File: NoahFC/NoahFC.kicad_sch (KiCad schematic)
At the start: 35 parts, among them J1 ALE, J10 GND, J11 SCK, J12 MISO, J13 VCC, J14 GND, J15 A1, J16 A3, J17 D6, J18 RESET, J2 ELE, J3 MPU6050, J4 FTDI, J5 VCC, J6 THR, J7 PPM, J8 GPS, J9 A0, U1 ATmega328, U3 AMS1117-5.0, Y1 16Mhz

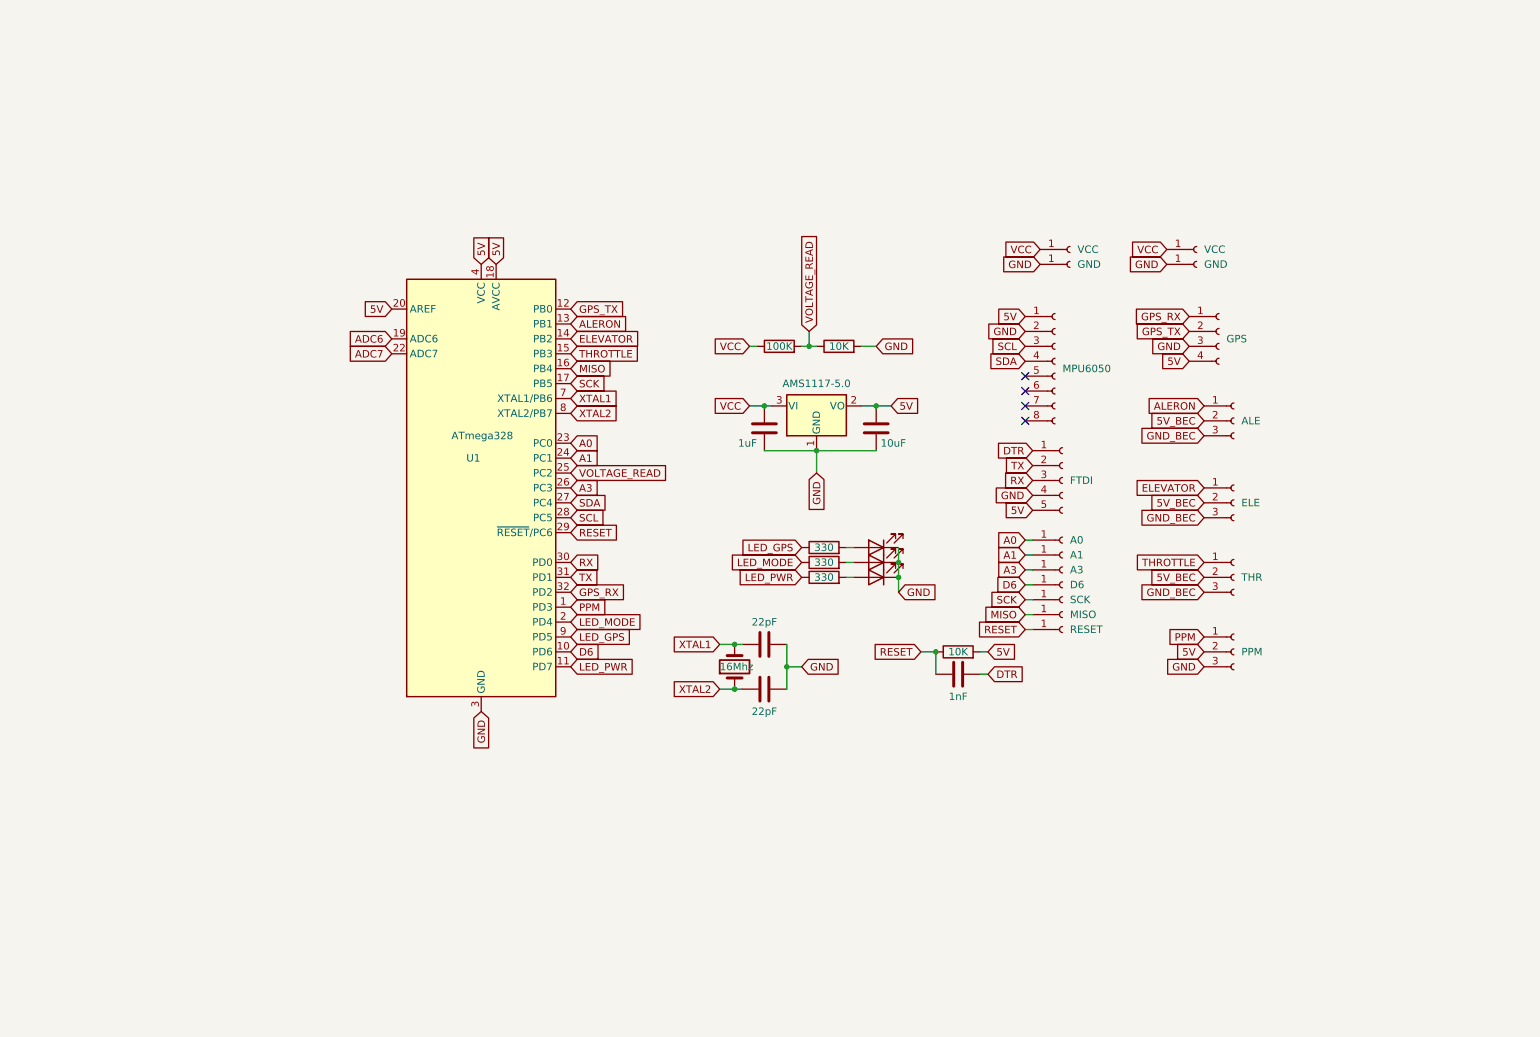
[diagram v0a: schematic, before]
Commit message: add rev2 version board
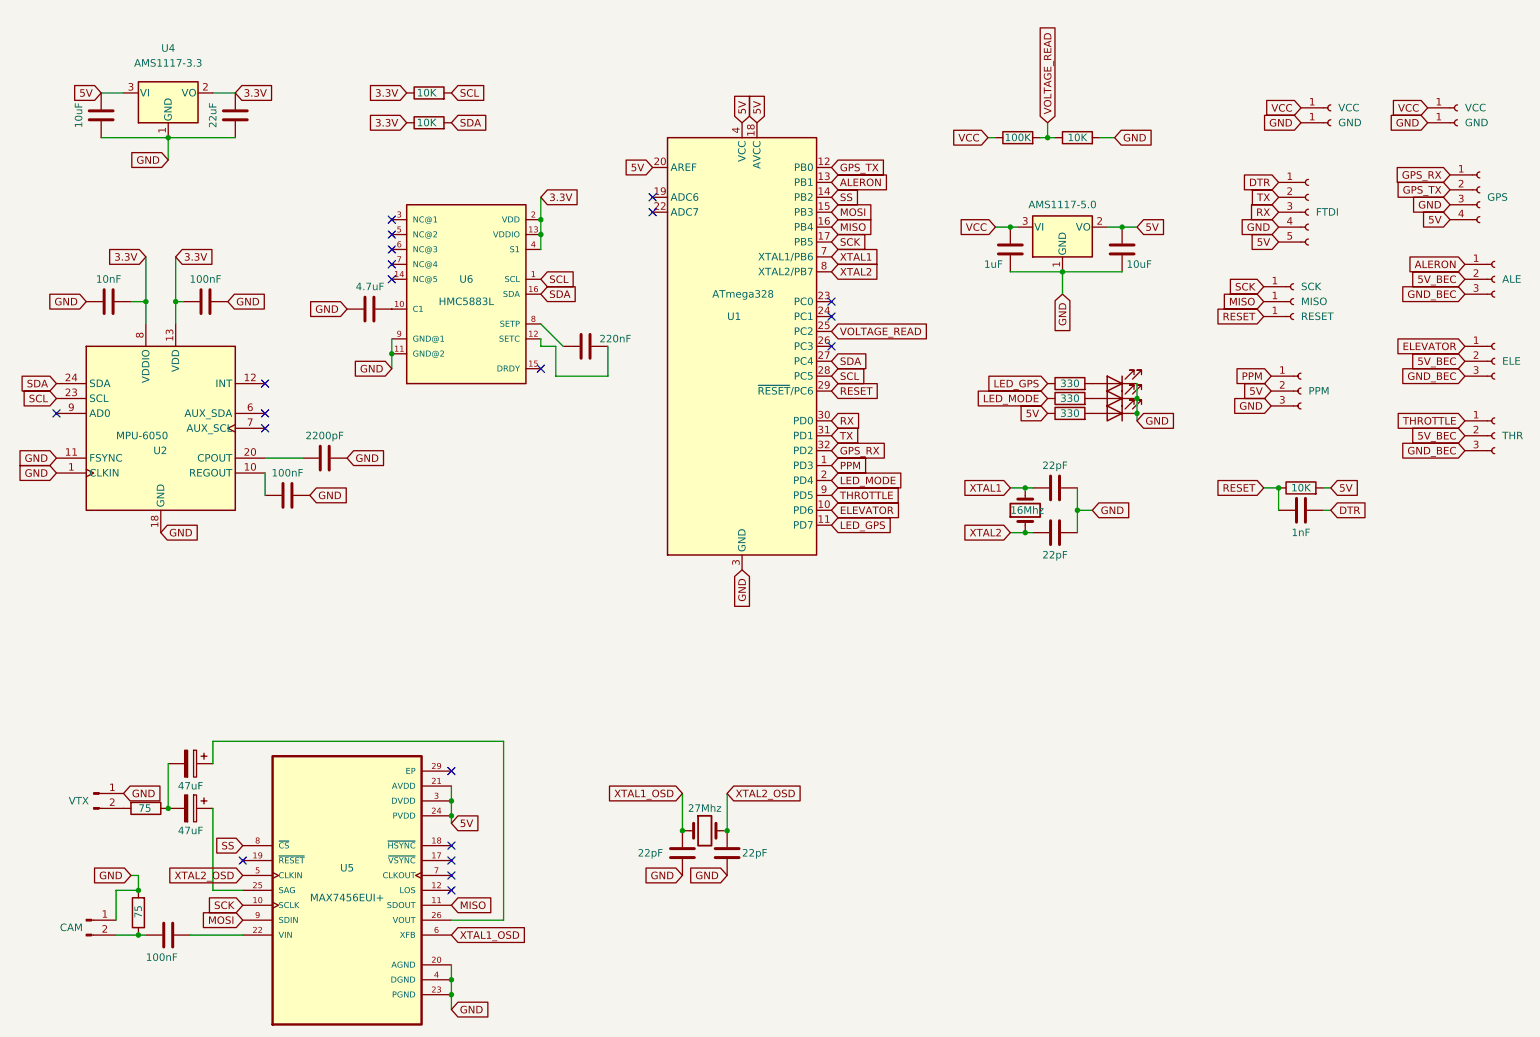
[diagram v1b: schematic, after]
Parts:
- removed J15: A1, TestPoint:TestPoint_Pad_1.0x1.0mm, symbol Connector:Conn_01x01_Female
- removed J16: A3, TestPoint:TestPoint_Pad_1.0x1.0mm, symbol Connector:Conn_01x01_Female
- removed J17: D6, TestPoint:TestPoint_Pad_1.0x1.0mm, symbol Connector:Conn_01x01_Female
- removed J3: MPU6050, Connector_PinHeader_2.54mm:PinHeader_1x08_P2.54mm_Vertical, symbol Connector:Conn_01x08_Female
- removed J9: A0, TestPoint:TestPoint_Pad_1.0x1.0mm, symbol Connector:Conn_01x01_Female
- added C10: 10uF, Capacitor_SMD:C_0805_2012Metric, symbol Device:C
- added C11: 22uF, Capacitor_SMD:C_0805_2012Metric, symbol Device:C
- added C12, C13: 22pF, Capacitor_SMD:C_0805_2012Metric, symbol Device:C
- added C17, C7, C8: 100nF, Capacitor_SMD:C_0805_2012Metric, symbol Device:C
- added C18, C19: 47uF, Capacitor_Tantalum_SMD:CP_EIA-3216-18_Kemet-A, symbol Device:C_Polarized
- added C20: 4.7uF, Capacitor_SMD:C_0805_2012Metric, symbol Device:C
- added C21: 220nF, Capacitor_SMD:C_0805_2012Metric, symbol Device:C
- added C6: 10nF, Capacitor_SMD:C_0805_2012Metric, symbol Device:C
- added C9: 2200pF, Capacitor_SMD:C_0805_2012Metric, symbol Device:C
- added J16: CAM, Connector_PinHeader_2.54mm:PinHeader_1x02_P2.54mm_Vertical, symbol Connector:Conn_01x02_Male
- added J17: VTX, Connector_PinHeader_2.54mm:PinHeader_1x02_P2.54mm_Vertical, symbol Connector:Conn_01x02_Male
- added R10, R9: 75, Resistor_SMD:R_0805_2012Metric, symbol Device:R
- added R7, R8: 10K, Resistor_SMD:R_0805_2012Metric, symbol Device:R
- added U2: MPU-6050, Sensor_Motion:InvenSense_QFN-24_4x4mm_P0.5mm, symbol Sensor_Motion:MPU-6050
- added U4: AMS1117-3.3, Package_TO_SOT_SMD:SOT-223-3_TabPin2, symbol Regulator_Linear:AP1117-33
- added U5: MAX7456EUI+, SOP65P637X110-28N, symbol MAX7456EUI_:MAX7456EUI+
- added U6: HMC5883L, LPCC-16, symbol HMC5883L:HMC5883L
- added Y2: 27Mhz, Crystal:Crystal_SMD_3225-4Pin_3.2x2.5mm, symbol Device:Crystal
- Y1: footprint Crystal:Crystal_SMD_HC49-SD -> Crystal:Crystal_SMD_3225-4Pin_3.2x2.5mm
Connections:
- net D6 is gone; now on net ELEVATOR: U1.10 (PD6)
- net 5V: now also R4.1, C10.2, U4.3 (VI), U5.21 (AVDD), U5.24 (PVDD), U5.3 (DVDD)
- net ELEVATOR: no longer U1.14 (PB2)
- net GND: now also C10.1, C11.1, C12.2, C13.2, C20.1, C6.1, C7.2, C8.2, C9.2, J16.1 (Pin_1), J17.1 (Pin_1), R9.2, U2.1 (CLKIN), U2.11 (FSYNC), U2.18 (GND), U4.1 (GND), U5.20 (AGND), U5.23 (PGND), U5.4 (DGND), U6.11 (GND@2), U6.9 (GND@1)
- net LED_GPS: now also U1.11 (PD7); no longer U1.9 (PD5)
- net MISO: now also U5.11 (SDOUT)
- net SCK: now also U5.10 (SCLK)
- net SCL: now also R7.2, U2.23 (SCL), U6.1 (SCL)
- net SDA: now also R8.2, U2.24 (SDA), U6.16 (SDA)
- net THROTTLE: now also U1.9 (PD5); no longer U1.15 (PB3)
- net A0: no longer names the net of U1.23 (PC0)
- net A1: no longer names the net of U1.24 (PC1)
- net A3: no longer names the net of U1.26 (PC3)
- net ADC6: no longer names the net of U1.19 (ADC6)
- net ADC7: no longer names the net of U1.22 (ADC7)
- removed net LED_PWR: R4.1, U1.11 (PD7)
- new net: C8.1, U2.10 (REGOUT)
- new net: C9.1, U2.20 (CPOUT)
- new net: C21.1, U6.8 (SETP)
- new net: C21.2, U6.12 (SETC)
- new net: C17.2, J16.2 (Pin_2), R9.1
- new net: C19.1, U5.26 (VOUT)
- new net: C18.2, C19.2, R10.1
- new net: C17.1, U5.22 (VIN)
- new net: J17.2 (Pin_2), R10.2
- new net: C20.2, U6.10 (C1)
- new net: C18.1, U5.25 (SAG)
- new net 3.3V: C11.2, C6.2, C7.1, R7.1, R8.1, U2.13 (VDD), U2.8 (VDDIO), U4.2 (VO), U6.13 (VDDIO), U6.2 (VDD), U6.4 (S1)
- new net MOSI: U1.15 (PB3), U5.9 (SDIN)
- new net SS: U1.14 (PB2), U5.8 (~{CS})
- new net XTAL1_OSD: C12.1, U5.6 (XFB), Y2.1
- new net XTAL2_OSD: C13.1, U5.5 (CLKIN), Y2.2
- no-connect marks 4 -> 21
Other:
- moved on the sheet: U1

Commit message: update scheme / design and board
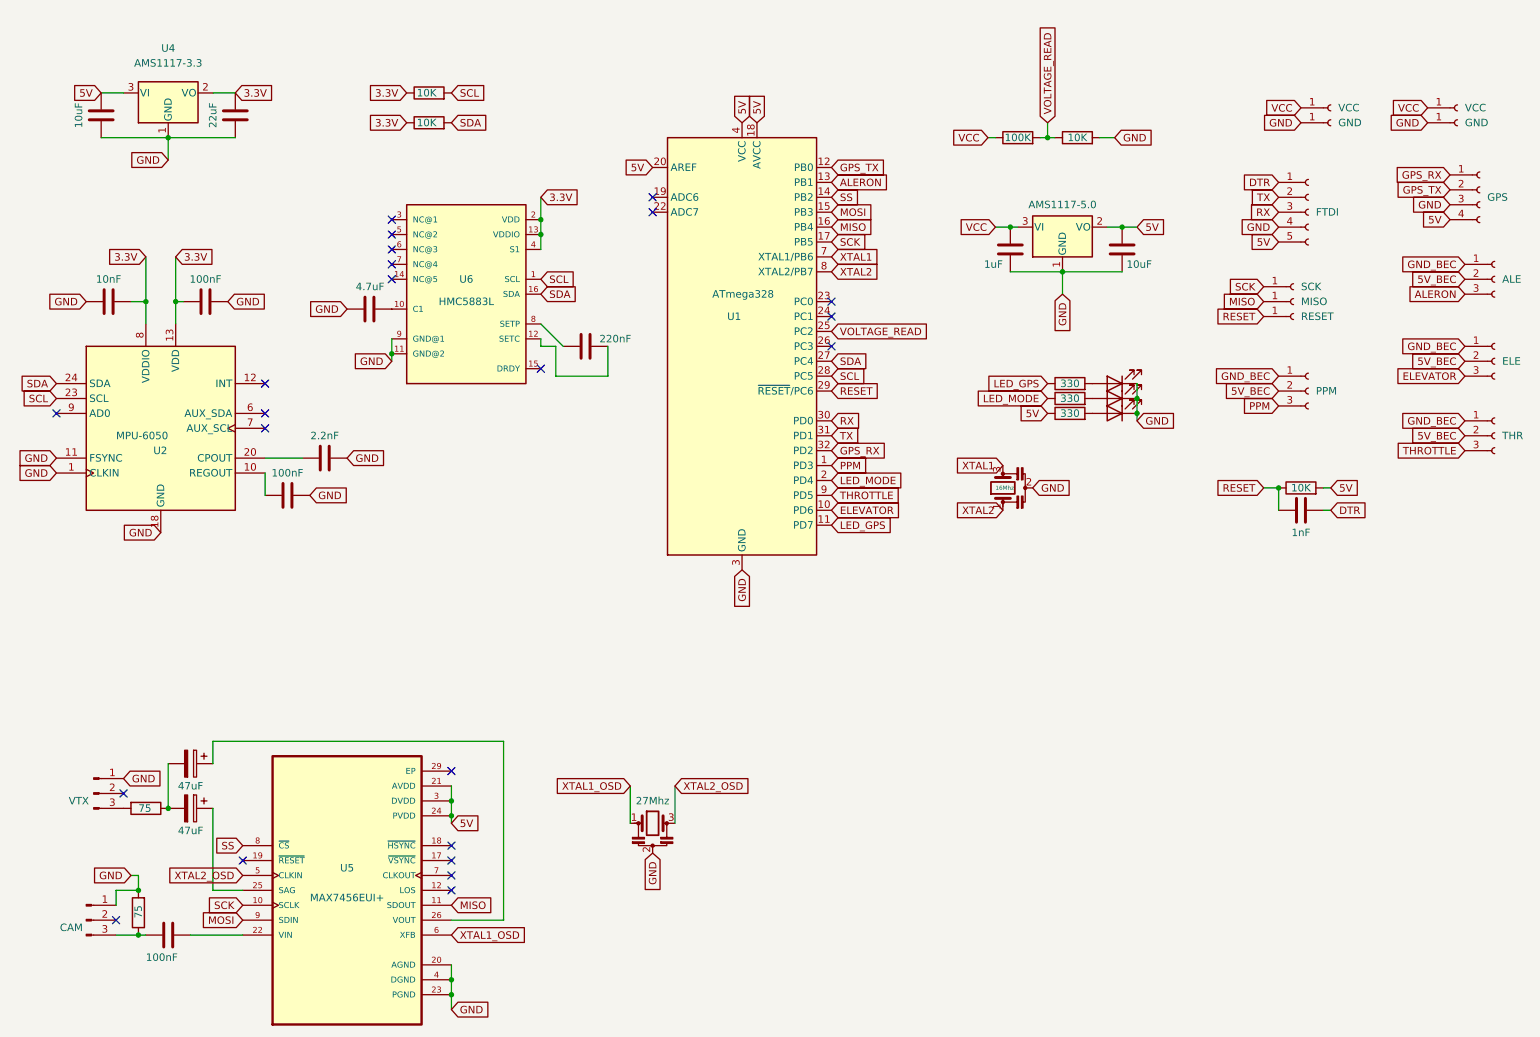
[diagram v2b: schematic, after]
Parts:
- removed C1, C12, C13, C2: 22pF, Capacitor_SMD:C_0805_2012Metric, symbol Device:C
- removed J16: CAM, Connector_PinHeader_2.54mm:PinHeader_1x02_P2.54mm_Vertical, symbol Connector:Conn_01x02_Male
- added J3: CAM, Connector_PinHeader_2.54mm:PinHeader_1x03_P2.54mm_Vertical, symbol Connector:Conn_01x03_Male
- C9: value 2200pF -> 2.2nF
- J17: footprint Connector_PinHeader_2.54mm:PinHeader_1x02_P2.54mm_Vertical -> Connector_PinHeader_2.54mm:PinHeader_1x03_P2.54mm_Vertical; symbol Connector:Conn_01x02_Male -> Connector:Conn_01x03_Male
- Y1: footprint Crystal:Crystal_SMD_3225-4Pin_3.2x2.5mm -> Crystal:Resonator_SMD_Murata_CSTxExxV-3Pin_3.0x1.1mm; symbol Device:Crystal -> Device:Resonator
- Y2: symbol Device:Crystal -> Device:Resonator
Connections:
- net 5V: no longer J7.2 (Pin_2)
- net 5V_BEC: now also J7.2 (Pin_2)
- net ALERON: now also J1.3 (Pin_3); no longer J1.1 (Pin_1)
- net ELEVATOR: now also J2.3 (Pin_3); no longer J2.1 (Pin_1)
- net GND: now also Y1.2, Y2.2, J3.1 (Pin_1); no longer J7.3 (Pin_3)
- net GND_BEC: now also J1.1 (Pin_1), J2.1 (Pin_1), J6.1 (Pin_1), J7.1 (Pin_1); no longer J1.3 (Pin_3), J2.3 (Pin_3), J6.3 (Pin_3)
- net PPM: now also J7.3 (Pin_3); no longer J7.1 (Pin_1)
- net THROTTLE: now also J6.3 (Pin_3); no longer J6.1 (Pin_1)
- net XTAL1: now also Y1.3; no longer Y1.2
- net XTAL2_OSD: now also Y2.3; no longer Y2.2
- net at C17.2, R9.1: now also J3.3 (Pin_3)
- net at J17.2 (Pin_2): no longer R10.2
- new net: J17.3 (Pin_3), R10.2
- no-connect marks 21 -> 23
